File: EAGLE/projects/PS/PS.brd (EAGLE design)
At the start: 73.6 x 43.5 mm, 5 parts

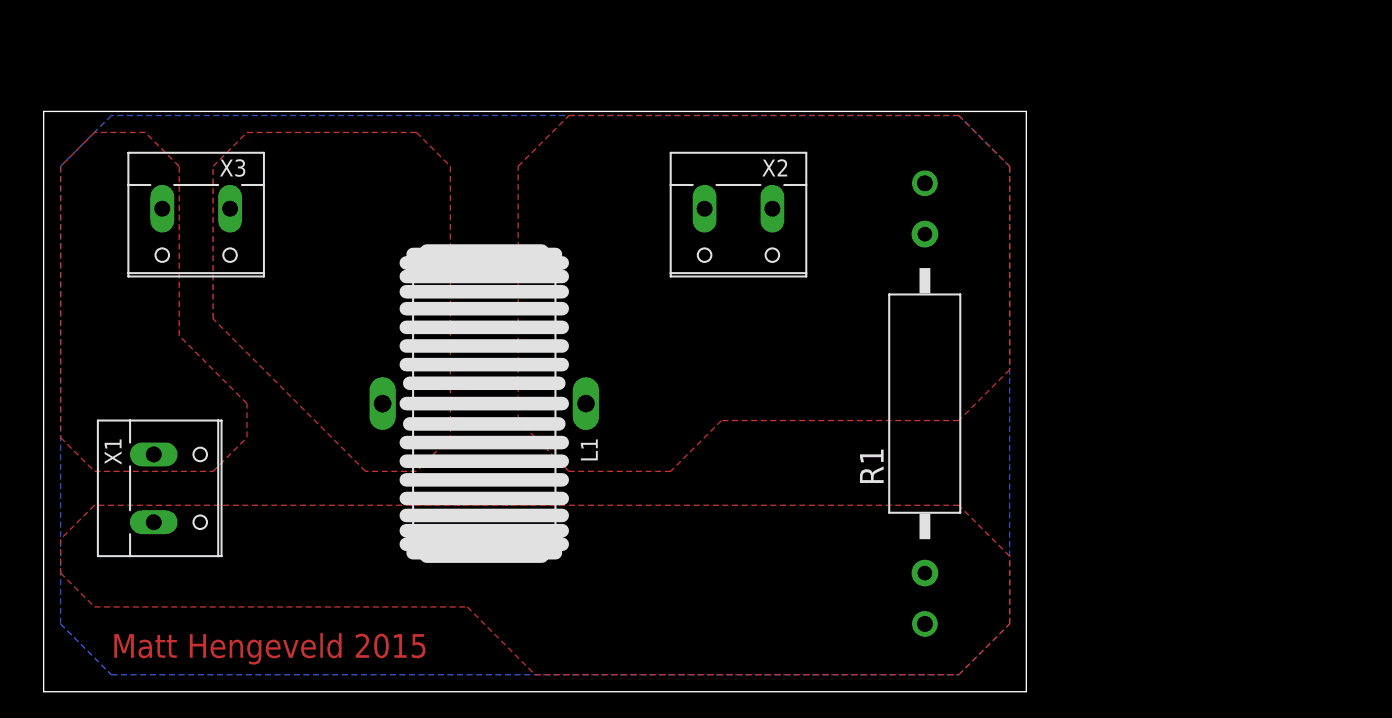
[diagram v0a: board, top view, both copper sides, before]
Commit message: changes
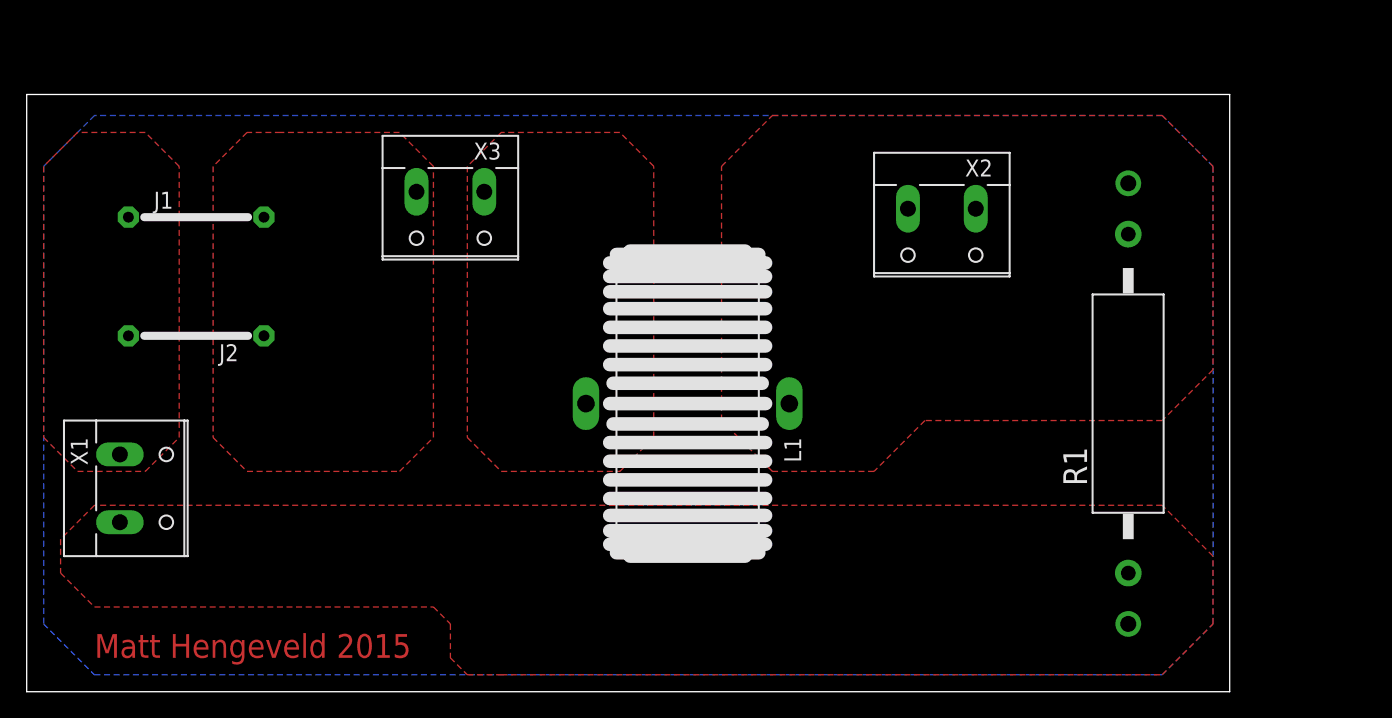
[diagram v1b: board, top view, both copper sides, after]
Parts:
- added J1, J2: J10MM, jumper:10
- moved X3 19.1 mm to (30.5, 36.8)
- moved X2 15.2 mm to (67.3, 35.6)
- moved L1 15.2 mm to (48.3, 21.6)
- moved R1 15.2 mm to (81.3, 21.6)
- moved X1 2.54 mm to (6.35, 15.2)
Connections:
- net VTHRU renamed VCAPS
- new net N$3: J1.2, J2.1, X3.2
- net VIN: now also J1.1, J2.2; no longer X3.2
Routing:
- added copper zone on layer 1, net N$3
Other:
- board size 73.6 x 43.5 mm -> 90.1 x 44.8 mm
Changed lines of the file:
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@@
 <board>
 <plain>
-<wire x1="0" y1="0" x2="73.64" y2="0" width="0" layer="20"/>
-<wire x1="73.64" y1="0" x2="73.64" y2="43.485" width="0" layer="20"/>
-<wire x1="73.64" y1="43.485" x2="0" y2="43.485" width="0" layer="20"/>
-<wire x1="0" y1="43.485" x2="0" y2="0" width="0" layer="20"/>
-<text x="5.08" y="2.54" size="1.778" layer="1">Matt Hengeveld 2015</text>
+<wire x1="-1.27" y1="0" x2="88.88" y2="0" width="0" layer="20"/>
+<wire x1="88.88" y1="0" x2="88.88" y2="44.755" width="0" layer="20"/>
+<wire x1="88.88" y1="44.755" x2="-1.27" y2="44.755" width="0" layer="20"/>
+<wire x1="-1.27" y1="44.755" x2="-1.27" y2="0" width="0" layer="20"/>
+<text x="3.81" y="2.54" size="1.778" layer="1">Matt Hengeveld 2015</text>
 </plain>
 <attributes>
@@
 </autorouter>
 <elements>
-<element name="X1" library="con-wago-508" package="W237-132" value="" x="8.89" y="15.24" rot="R270">
-<attribute name="OC_NEWARK" value="unknown" x="-19.05" y="-3.81" size="1.778" layer="27" rot="R270" display="off"/>
-<attribute name="MPN" value="" x="-19.05" y="-3.81" size="1.778" layer="27" rot="R270" display="off"/>
-<attribute name="MF" value="" x="-19.05" y="-3.81" size="1.778" layer="27" rot="R270" display="off"/>
-<attribute name="OC_FARNELL" value="unknown" x="-19.05" y="-3.81" size="1.778" layer="27" rot="R270" display="off"/>
+<element name="X1" library="con-wago-508" package="W237-132" value="" x="6.35" y="15.24" rot="R270">
+<attribute name="OC_NEWARK" value="unknown" x="-21.59" y="-3.81" size="1.778" layer="27" rot="R270" display="off"/>
+<attribute name="MPN" value="" x="-21.59" y="-3.81" size="1.778" layer="27" rot="R270" display="off"/>
+<attribute name="MF" value="" x="-21.59" y="-3.81" size="1.778" layer="27" rot="R270" display="off"/>
+<attribute name="OC_FARNELL" value="unknown" x="-21.59" y="-3.81" size="1.778" layer="27" rot="R270" display="off"/>
 </element>
-<element name="X2" library="con-wago-508" package="W237-132" value="" x="52.07" y="35.56" rot="R180">
-<attribute name="OC_NEWARK" value="unknown" x="21.59" y="63.5" size="1.778" layer="27" rot="R180" display="off"/>
-<attribute name="MPN" value="" x="21.59" y="63.5" size="1.778" layer="27" rot="R180" display="off"/>
-<attribute name="MF" value="" x="21.59" y="63.5" size="1.778" layer="27" rot="R180" display="off"/>
-<attribute name="OC_FARNELL" value="unknown" x="21.59" y="63.5" size="1.778" layer="27" rot="R180" display="off"/>
+<element name="X2" library="con-wago-508" package="W237-132" value="" x="67.31" y="35.56" rot="R180">
+<attribute name="OC_NEWARK" value="unknown" x="36.83" y="63.5" size="1.778" layer="27" rot="R180" display="off"/>
+<attribute name="MPN" value="" x="36.83" y="63.5" size="1.778" layer="27" rot="R180" display="off"/>
+<attribute name="MF" value="" x="36.83" y="63.5" size="1.778" layer="27" rot="R180" display="off"/>
+<attribute name="OC_FARNELL" value="unknown" x="36.83" y="63.5" size="1.778" layer="27" rot="R180" display="off"/>
 </element>
-<element name="L1" library="inductors" package="SFT1240" value="SFT1240" x="33.02" y="21.59" rot="R180"/>
-<element name="X3" library="con-wago-508" package="W237-132" value="" x="11.43" y="35.56" rot="R180">
-<attribute name="OC_NEWARK" value="unknown" x="11.43" y="35.56" size="1.778" layer="27" rot="R180" display="off"/>
-<attribute name="MPN" value="" x="11.43" y="35.56" size="1.778" layer="27" rot="R180" display="off"/>
-<attribute name="MF" value="" x="11.43" y="35.56" size="1.778" layer="27" rot="R180" display="off"/>
-<attribute name="OC_FARNELL" value="unknown" x="11.43" y="35.56" size="1.778" layer="27" rot="R180" display="off"/>
+<element name="L1" library="inductors" package="SFT1240" value="SFT1240" x="48.26" y="21.59" rot="R180"/>
+<element name="X3" library="con-wago-508" package="W237-132" value="" x="30.48" y="36.83" rot="R180">
+<attribute name="OC_NEWARK" value="unknown" x="30.48" y="36.83" size="1.778" layer="27" rot="R180" display="off"/>
+<attribute name="MPN" value="" x="30.48" y="36.83" size="1.778" layer="27" rot="R180" display="off"/>
+<attribute name="MF" value="" x="30.48" y="36.83" size="1.778" layer="27" rot="R180" display="off"/>
+<attribute name="OC_FARNELL" value="unknown" x="30.48" y="36.83" size="1.778" layer="27" rot="R180" display="off"/>
 </element>
-<element name="R1" library="resistor-power" package="AC04" value="" x="66.04" y="21.59" rot="R90">
-<attribute name="OC_NEWARK" value="unknown" x="66.04" y="21.59" size="1.778" layer="27" rot="R90" display="off"/>
-<attribute name="MPN" value="" x="66.04" y="21.59" size="1.778" layer="27" rot="R90" display="off"/>
-<attribute name="MF" value="" x="66.04" y="21.59" size="1.778" layer="27" rot="R90" display="off"/>
-<attribute name="OC_FARNELL" value="unknown" x="66.04" y="21.59" size="1.778" layer="27" rot="R90" display="off"/>
+<element name="R1" library="resistor-power" package="AC04" value="" x="81.28" y="21.59" rot="R90">
+<attribute name="OC_NEWARK" value="unknown" x="81.28" y="21.59" size="1.778" layer="27" rot="R90" display="off"/>
+<attribute name="MPN" value="" x="81.28" y="21.59" size="1.778" layer="27" rot="R90" display="off"/>
+<attribute name="MF" value="" x="81.28" y="21.59" size="1.778" layer="27" rot="R90" display="off"/>
+<attribute name="OC_FARNELL" value="unknown" x="81.28" y="21.59" size="1.778" layer="27" rot="R90" display="off"/>
 </element>
+<element name="J1" library="jumper" package="10" value="J10MM" x="11.43" y="35.56"/>
+<element name="J2" library="jumper" package="10" value="J10MM" x="11.43" y="26.67" rot="R180"/>
 </elements>
 <signals>
@@
 <contactref element="R1" pad="2"/>
 <polygon width="0.4064" layer="1" thermals="no">
-<vertex x="39.37" y="16.51"/>
-<vertex x="35.56" y="20.32"/>
-<vertex x="35.56" y="39.37"/>
-<vertex x="39.37" y="43.18"/>
-<vertex x="68.58" y="43.18"/>
-<vertex x="72.39" y="39.37"/>
-<vertex x="72.39" y="24.13"/>
-<vertex x="68.58" y="20.32"/>
+<vertex x="54.61" y="16.51"/>
 <vertex x="50.8" y="20.32"/>
-<vertex x="46.99" y="16.51"/>
+<vertex x="50.8" y="39.37"/>
+<vertex x="54.61" y="43.18"/>
+<vertex x="83.82" y="43.18"/>
+<vertex x="87.63" y="39.37"/>
+<vertex x="87.63" y="24.13"/>
+<vertex x="83.82" y="20.32"/>
+<vertex x="66.04" y="20.32"/>
+<vertex x="62.23" y="16.51"/>
 </polygon>
 <contactref element="X2" pad="2"/>
-<via x="66.04" y="38.1" extent="1-16" drill="1.2" diameter="1.9304"/>
+<via x="81.28" y="38.1" extent="1-16" drill="1.2" diameter="1.9304"/>
 </signal>
 <signal name="GND">
 <polygon width="0.4064" layer="16" isolate="1.778" thermals="no">
-<vertex x="25.4" y="43.18"/>
-<vertex x="5.08" y="43.18"/>
-<vertex x="1.27" y="39.37"/>
-<vertex x="1.27" y="5.08"/>
-<vertex x="5.08" y="1.27"/>
-<vertex x="68.58" y="1.27"/>
-<vertex x="72.39" y="5.08"/>
-<vertex x="72.39" y="39.37"/>
-<vertex x="68.58" y="43.18"/>
-</polygon>
-<contactref element="X1" pad="2"/>
+<vertex x="83.82" y="43.18"/>
+<vertex x="3.81" y="43.18"/>
+<vertex x="0" y="39.37"/>
+<vertex x="0" y="5.08"/>
+<vertex x="3.81" y="1.27"/>
+<vertex x="83.82" y="1.27"/>
+<vertex x="87.63" y="5.08"/>
+<vertex x="87.63" y="39.37"/>
+</polygon>
 <contactref element="X2" pad="1"/>
 <contactref element="R1" pad="1"/>
@@
 <vertex x="1.27" y="8.89"/>
 <vertex x="3.81" y="6.35"/>
-<vertex x="31.75" y="6.35"/>
-<vertex x="36.83" y="1.27"/>
-<vertex x="68.58" y="1.27"/>
-<vertex x="72.39" y="5.08"/>
-<vertex x="72.39" y="10.16"/>
-<vertex x="68.58" y="13.97"/>
-</polygon>
-<via x="66.04" y="5.08" extent="1-16" drill="1.2" diameter="1.9304"/>
+<vertex x="29.21" y="6.35"/>
+<vertex x="30.48" y="5.08"/>
+<vertex x="30.48" y="2.54"/>
+<vertex x="31.75" y="1.27"/>
+<vertex x="34.29" y="1.27"/>
+<vertex x="83.82" y="1.27"/>
+<vertex x="87.63" y="5.08"/>
+<vertex x="87.63" y="10.16"/>
+<vertex x="83.82" y="13.97"/>
+</polygon>
+<via x="81.28" y="5.08" extent="1-16" drill="1.2" diameter="1.9304"/>
+<contactref element="X1" pad="2"/>
 </signal>
 <signal name="VIN">
-<contactref element="X1" pad="1"/>
-<contactref element="X3" pad="2"/>
 <polygon width="0.4064" layer="1" thermals="no">
 <vertex x="10.16" y="39.37"/>
 <vertex x="7.62" y="41.91"/>
-<vertex x="3.81" y="41.91"/>
-<vertex x="1.27" y="39.37"/>
-<vertex x="1.27" y="19.05"/>
-<vertex x="3.81" y="16.51"/>
-<vertex x="12.7" y="16.51"/>
-<vertex x="15.24" y="19.05"/>
-<vertex x="15.24" y="21.59"/>
-<vertex x="10.16" y="26.67"/>
-</polygon>
-</signal>
-<signal name="VTHRU">
+<vertex x="2.54" y="41.91"/>
+<vertex x="0" y="39.37"/>
+<vertex x="0" y="19.05"/>
+<vertex x="2.54" y="16.51"/>
+<vertex x="7.62" y="16.51"/>
+<vertex x="10.16" y="19.05"/>
+</polygon>
+<contactref element="J2" pad="2"/>
+<contactref element="J1" pad="1"/>
+<contactref element="X1" pad="1"/>
+</signal>
+<signal name="VCAPS">
 <contactref element="X3" pad="1"/>
 <contactref element="L1" pad="2"/>
-<polygon width="0.4064" layer="1" thermals="no">
-<vertex x="27.94" y="16.51"/>
-<vertex x="24.13" y="16.51"/>
-<vertex x="12.7" y="27.94"/>
+<polygon width="0.4064" layer="1" isolate="1.016" thermals="no">
+<vertex x="34.29" y="41.91"/>
+<vertex x="31.75" y="39.37"/>
+<vertex x="31.75" y="19.05"/>
+<vertex x="34.29" y="16.51"/>
+<vertex x="43.18" y="16.51"/>
+<vertex x="45.72" y="19.05"/>
+<vertex x="45.72" y="39.37"/>
+<vertex x="43.18" y="41.91"/>
+</polygon>
+<wire x1="40.64" y1="21.59" x2="33.02" y2="37.465" width="0" layer="19" extent="1-1"/>
+</signal>
+<signal name="N$3">
+<contactref element="J1" pad="2"/>
+<contactref element="X3" pad="2"/>
+<contactref element="J2" pad="1"/>
+<polygon width="0.4064" layer="1" isolate="1.016" thermals="no">
+<vertex x="17.78" y="41.91"/>
+<vertex x="15.24" y="41.91"/>
 <vertex x="12.7" y="39.37"/>
-<vertex x="15.24" y="41.91"/>
-<vertex x="27.94" y="41.91"/>
-<vertex x="30.48" y="39.37"/>
-<vertex x="30.48" y="19.05"/>
-</polygon>
-</signal>
+<vertex x="12.7" y="19.05"/>
+<vertex x="15.24" y="16.51"/>
+<vertex x="26.67" y="16.51"/>
+<vertex x="29.21" y="19.05"/>
+<vertex x="29.21" y="39.37"/>
+<vertex x="26.67" y="41.91"/>
+</polygon>
+</signal>

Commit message: a lot
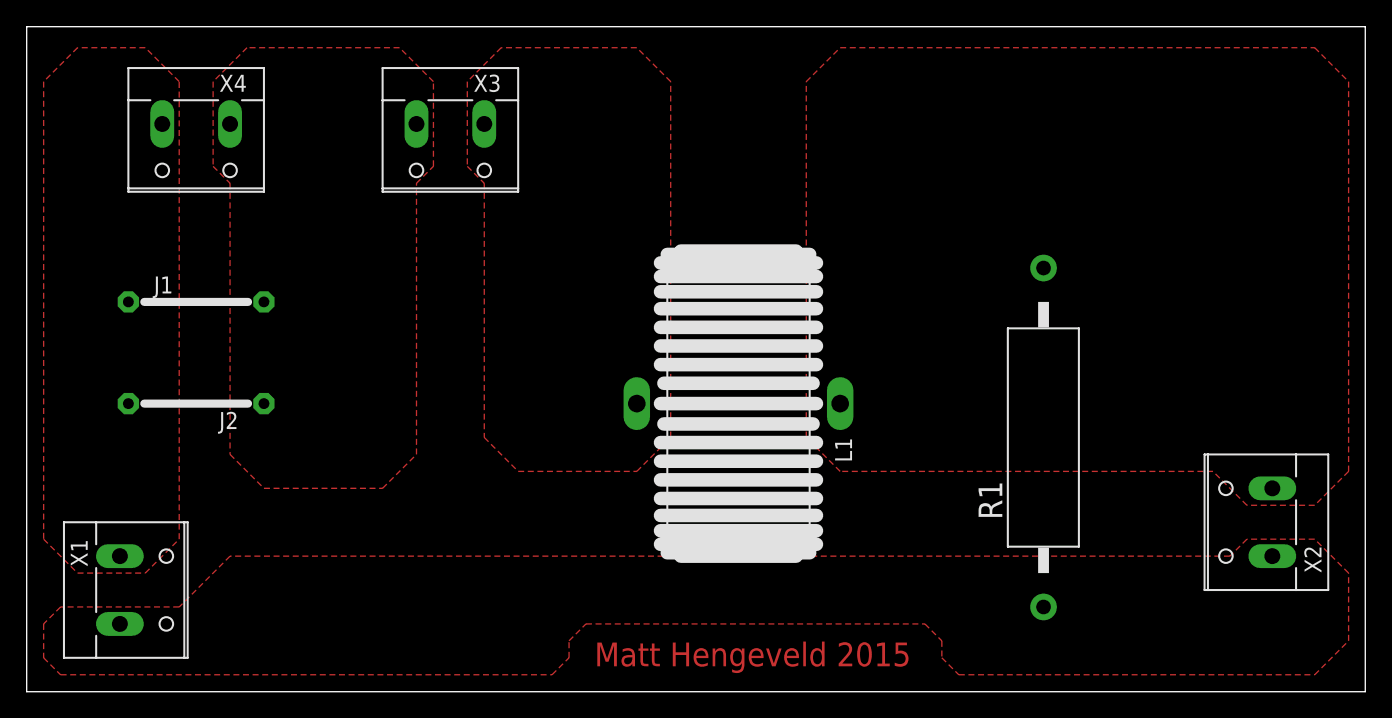
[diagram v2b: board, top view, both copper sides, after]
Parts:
- added X4: (no value), con-wago-508:W237-132
- moved X2 33.2 mm to (91.4, 12.7), turned to 90 degrees
- moved X1 7.62 mm to (6.35, 7.62)
- moved R1 6.84 mm to (74.9, 19.1)
- moved J1 6.35 mm to (11.4, 29.2)
- moved J2 5.08 mm to (11.4, 21.6)
- moved X3 5.08 mm to (30.5, 41.9)
- moved L1 3.81 mm to (52.1, 21.6)
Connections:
- net N$3: now also X4.1
- net VIN: now also X4.2
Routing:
- removed copper zone on layer 16, net GND
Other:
- board size 90.1 x 44.8 mm -> 100.3 x 49.8 mm
